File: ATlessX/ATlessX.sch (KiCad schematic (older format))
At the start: 13 parts, among them U1 74LS74, U2 74LS14

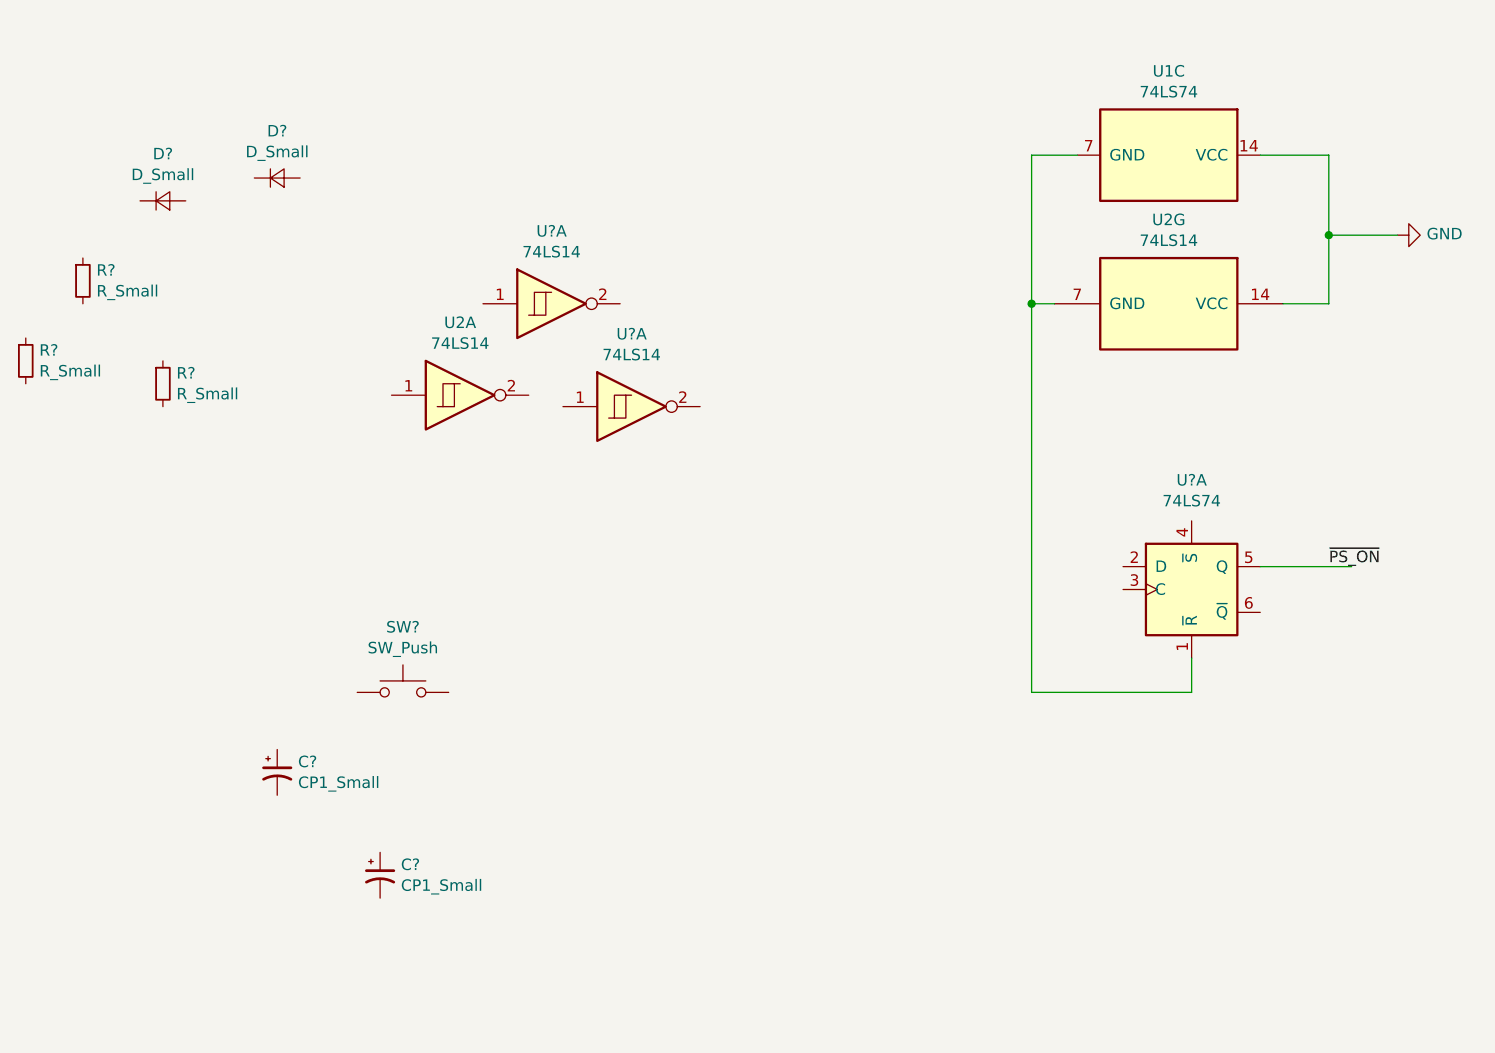
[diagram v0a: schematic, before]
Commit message: More of the circuit done
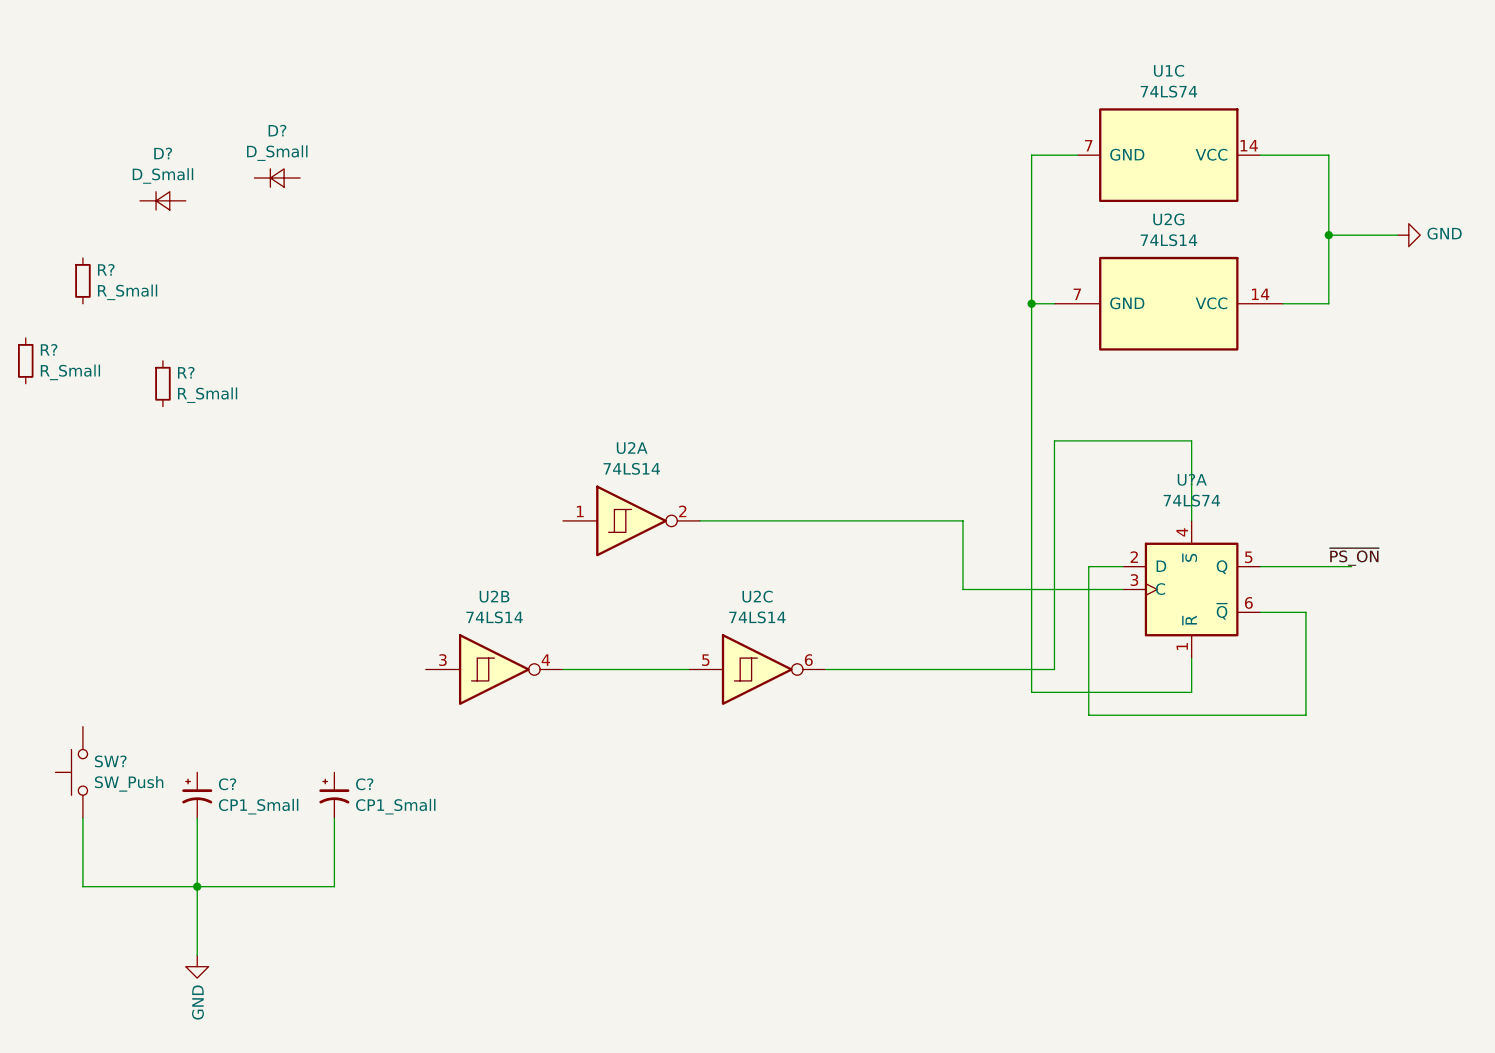
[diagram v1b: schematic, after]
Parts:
- gave numbers to parts that had none: 1
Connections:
- wire segments 12 -> 31
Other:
- moved on the sheet: C?, SW?, U2A
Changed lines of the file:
@@
 $Comp
 L 74xx:74LS14 U2
-U 1 1 5DD82518
-P 2500 2300
-F 0 "U2" H 2500 2617 50  0000 C CNN
-F 1 "74LS14" H 2500 2526 50  0000 C CNN
-F 2 "" H 2500 2300 50  0001 C CNN
-F 3 "http://www.ti.com/lit/gpn/sn74LS14" H 2500 2300 50  0001 C CNN
-	1    2500 2300
+U 2 1 5DD82518
+P 2650 3500
+F 0 "U2" H 2650 3817 50  0000 C CNN
+F 1 "74LS14" H 2650 3726 50  0000 C CNN
+F 2 "" H 2650 3500 50  0001 C CNN
+F 3 "http://www.ti.com/lit/gpn/sn74LS14" H 2650 3500 50  0001 C CNN
+	2    2650 3500
 	1    0    0    -1
 $EndComp
@@
 L Switch:SW_Push SW?
 U 1 1 5DD82728
-P 2250 3600
-F 0 "SW?" H 2250 3885 50  0000 C CNN
-F 1 "SW_Push" H 2250 3794 50  0000 C CNN
-F 2 "" H 2250 3800 50  0001 C CNN
-F 3 "~" H 2250 3800 50  0001 C CNN
-	1    2250 3600
-	1    0    0    -1
+P 850 3950
+F 0 "SW?" V 896 3902 50  0000 R CNN
+F 1 "SW_Push" V 805 3902 50  0000 R CNN
+F 2 "" H 850 4150 50  0001 C CNN
+F 3 "~" H 850 4150 50  0001 C CNN
+	1    850  3950
+	0    -1   -1   0
 $EndComp
 $Comp
 L Device:CP1_Small C?
 U 1 1 5DD82992
-P 2150 4400
-F 0 "C?" H 2241 4446 50  0000 L CNN
-F 1 "CP1_Small" H 2241 4355 50  0000 L CNN
-F 2 "" H 2150 4400 50  0001 C CNN
-F 3 "~" H 2150 4400 50  0001 C CNN
-	1    2150 4400
-	1    0    0    -1
-$EndComp
-$Comp
-L 74xx:74LS14 U?
+P 1950 4050
+F 0 "C?" H 2041 4096 50  0000 L CNN
+F 1 "CP1_Small" H 2041 4005 50  0000 L CNN
+F 2 "" H 1950 4050 50  0001 C CNN
+F 3 "~" H 1950 4050 50  0001 C CNN
+	1    1950 4050
+	1    0    0    -1
+$EndComp
+$Comp
+L 74xx:74LS14 U2
 U 1 1 5DD82CD4
-P 2900 1900
-F 0 "U?" H 2900 2217 50  0000 C CNN
-F 1 "74LS14" H 2900 2126 50  0000 C CNN
-F 2 "" H 2900 1900 50  0001 C CNN
-F 3 "http://www.ti.com/lit/gpn/sn74LS14" H 2900 1900 50  0001 C CNN
-	1    2900 1900
-	1    0    0    -1
-$EndComp
-$Comp
-L 74xx:74LS14 U?
-U 1 1 5DD82D12
-P 3250 2350
-F 0 "U?" H 3250 2667 50  0000 C CNN
-F 1 "74LS14" H 3250 2576 50  0000 C CNN
-F 2 "" H 3250 2350 50  0001 C CNN
-F 3 "http://www.ti.com/lit/gpn/sn74LS14" H 3250 2350 50  0001 C CNN
-	1    3250 2350
+P 3250 2850
+F 0 "U2" H 3250 3167 50  0000 C CNN
+F 1 "74LS14" H 3250 3076 50  0000 C CNN
+F 2 "" H 3250 2850 50  0001 C CNN
+F 3 "http://www.ti.com/lit/gpn/sn74LS14" H 3250 2850 50  0001 C CNN
+	1    3250 2850
+	1    0    0    -1
+$EndComp
+$Comp
+L 74xx:74LS14 U2
+U 3 1 5DD82D12
+P 3800 3500
+F 0 "U2" H 3800 3817 50  0000 C CNN
+F 1 "74LS14" H 3800 3726 50  0000 C CNN
+F 2 "" H 3800 3500 50  0001 C CNN
+F 3 "http://www.ti.com/lit/gpn/sn74LS14" H 3800 3500 50  0001 C CNN
+	3    3800 3500
 	1    0    0    -1
 $EndComp
@@
 L Device:CP1_Small C?
 U 1 1 5DD82E48
-P 1700 3950
-F 0 "C?" H 1791 3996 50  0000 L CNN
-F 1 "CP1_Small" H 1791 3905 50  0000 L CNN
-F 2 "" H 1700 3950 50  0001 C CNN
-F 3 "~" H 1700 3950 50  0001 C CNN
-	1    1700 3950
-	1    0    0    -1
-$EndComp
+P 1350 4050
+F 0 "C?" H 1441 4096 50  0000 L CNN
+F 1 "CP1_Small" H 1441 4005 50  0000 L CNN
+F 2 "" H 1350 4050 50  0001 C CNN
+F 3 "~" H 1350 4050 50  0001 C CNN
+	1    1350 4050
+	1    0    0    -1
+$EndComp
+Wire Wire Line
+	2950 3500 3500 3500
+Wire Wire Line
+	4100 3500 5100 3500
+Wire Wire Line
+	5100 3500 5100 2500
+Wire Wire Line
+	5100 2500 5700 2500
+Wire Wire Line
+	5700 2500 5700 2850
+Wire Wire Line
+	3550 2850 4700 2850
+Wire Wire Line
+	4700 2850 4700 3150
+Wire Wire Line
+	4700 3150 5400 3150
+Wire Wire Line
+	5400 3050 5250 3050
+Wire Wire Line
+	5250 3050 5250 3700
+Wire Wire Line
+	5250 3700 6200 3700
+Wire Wire Line
+	6200 3700 6200 3250
+Wire Wire Line
+	6200 3250 6000 3250
+Wire Wire Line
+	850  4150 850  4450
+Wire Wire Line
+	850  4450 1350 4450
+Wire Wire Line
+	1950 4450 1950 4150
+Wire Wire Line
+	1350 4150 1350 4450
+Connection ~ 1350 4450
+Wire Wire Line
+	1350 4450 1950 4450
+$Comp
+L power:GND #PWR?
+U 1 1 5DD84F2D
+P 1350 4750
+F 0 "#PWR?" H 1350 4500 50  0001 C CNN
+F 1 "GND" V 1355 4622 50  0000 R CNN
+F 2 "" H 1350 4750 50  0001 C CNN
+F 3 "" H 1350 4750 50  0001 C CNN
+	1    1350 4750
+	1    0    0    -1
+$EndComp
+Wire Wire Line
+	1350 4450 1350 4750
 $EndSCHEMATC

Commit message: Update schematic
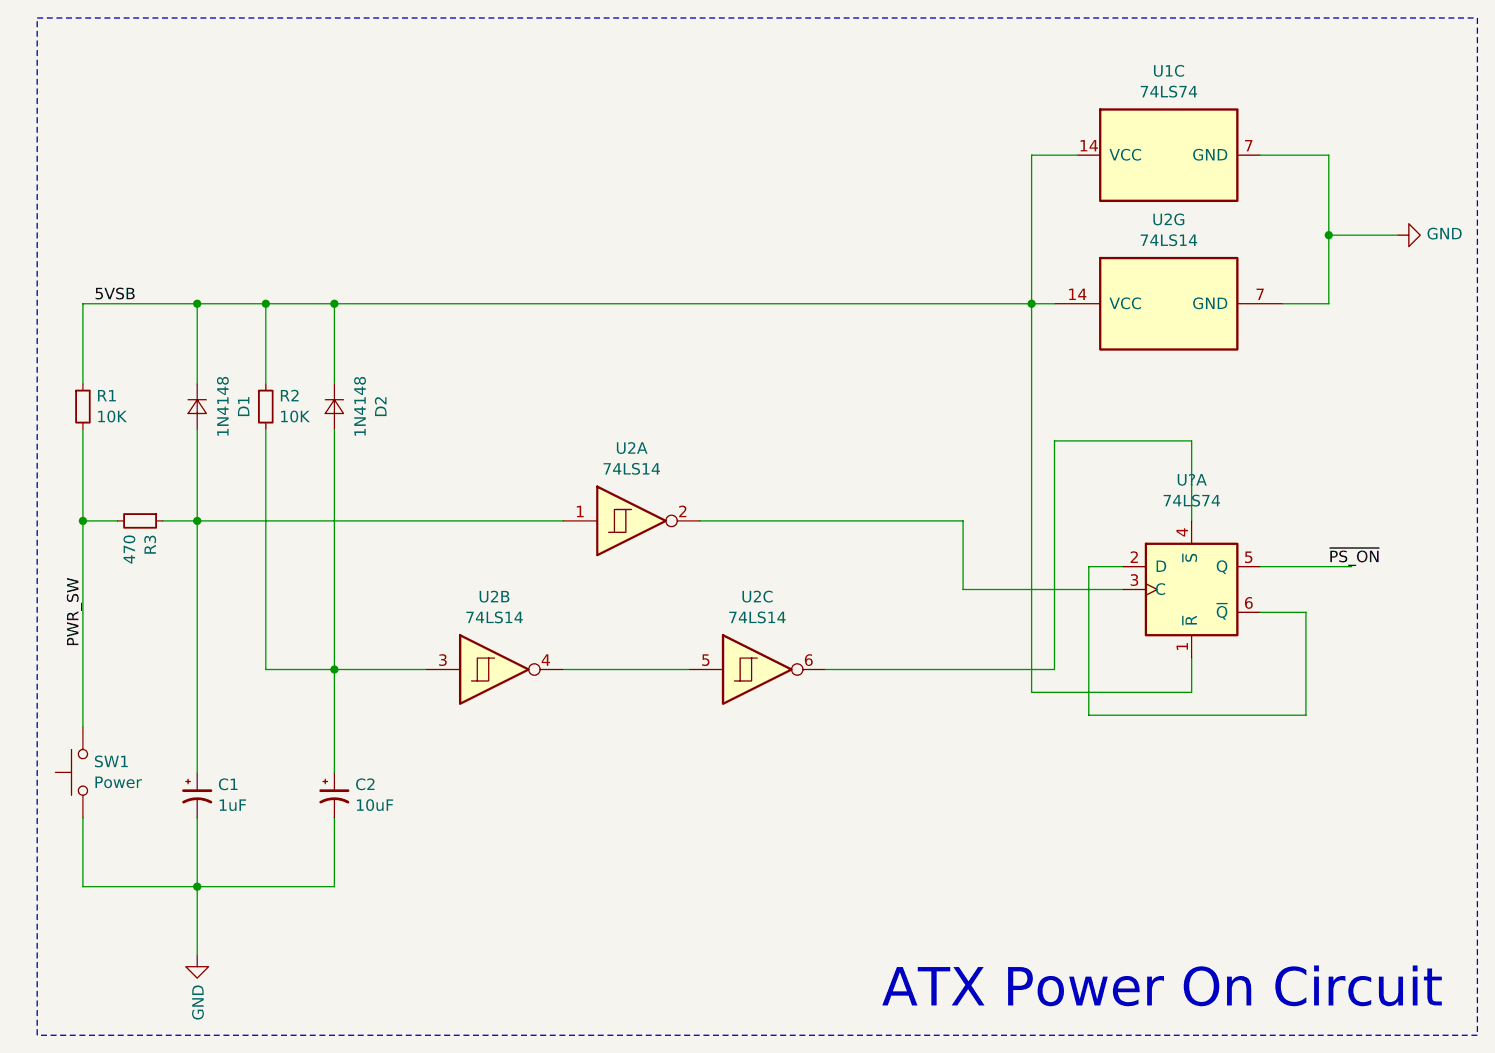
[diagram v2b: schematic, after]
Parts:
- C1: renamed from C?; value CP1_Small -> 1uF
- C2: renamed from C?; value CP1_Small -> 10uF
- D1, D2: renamed from D?; value D_Small -> 1N4148
- R1, R2: renamed from R?; value R_Small -> 10K
- R3: renamed from R?; value R_Small -> 470
- SW1: renamed from SW?; value SW_Push -> Power
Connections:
- net labels added: 5VSB, PWR_SW
- wire segments 31 -> 51
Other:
- note added: "ATX Power On Circuit"
- moved on the sheet: D1, D2, R1, R2, R3
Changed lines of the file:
@@
 F 3 "74xx/74hc_hct74.pdf" H 5600 1250 50  0001 C CNN
 	3    5600 1250
-	0    1    1    0
+	0    -1   1    0
 $EndComp
 $Comp
@@
 F 3 "http://www.ti.com/lit/gpn/sn74LS14" H 5600 1900 50  0001 C CNN
 	7    5600 1900
-	0    1    1    0
+	0    -1   1    0
 $EndComp
 Wire Wire Line
@@
 Connection ~ 5000 1900
 $Comp
-L Device:D_Small D?
+L Device:D_Small D1
 U 1 1 5DD82675
-P 1200 1450
-F 0 "D?" H 1200 1655 50  0000 C CNN
-F 1 "D_Small" H 1200 1564 50  0000 C CNN
-F 2 "" V 1200 1450 50  0001 C CNN
-F 3 "~" V 1200 1450 50  0001 C CNN
-	1    1200 1450
-	1    0    0    -1
-$EndComp
-$Comp
-L Device:R_Small R?
+P 1350 2350
+F 0 "D1" H 1350 2555 50  0000 C CNN
+F 1 "1N4148" H 1350 2464 50  0000 C CNN
+F 2 "" V 1350 2350 50  0001 C CNN
+F 3 "~" V 1350 2350 50  0001 C CNN
+	1    1350 2350
+	0    1    1    0
+$EndComp
+$Comp
+L Device:R_Small R3
 U 1 1 5DD827BB
-P 850 1800
-F 0 "R?" H 909 1846 50  0000 L CNN
-F 1 "R_Small" H 909 1755 50  0000 L CNN
-F 2 "" H 850 1800 50  0001 C CNN
-F 3 "~" H 850 1800 50  0001 C CNN
-	1    850  1800
-	1    0    0    -1
-$EndComp
-$Comp
-L Switch:SW_Push SW?
+P 1100 2850
+F 0 "R3" H 1159 2896 50  0000 L CNN
+F 1 "470" H 1159 2805 50  0000 L CNN
+F 2 "" H 1100 2850 50  0001 C CNN
+F 3 "~" H 1100 2850 50  0001 C CNN
+	1    1100 2850
+	0    1    1    0
+$EndComp
+$Comp
+L Switch:SW_Push SW1
 U 1 1 5DD82728
 P 850 3950
-F 0 "SW?" V 896 3902 50  0000 R CNN
-F 1 "SW_Push" V 805 3902 50  0000 R CNN
+F 0 "SW1" V 896 3902 50  0000 R CNN
+F 1 "Power" V 805 3902 50  0000 R CNN
 F 2 "" H 850 4150 50  0001 C CNN
 F 3 "~" H 850 4150 50  0001 C CNN
@@
 $EndComp
 $Comp
-L Device:CP1_Small C?
+L Device:CP1_Small C2
 U 1 1 5DD82992
 P 1950 4050
-F 0 "C?" H 2041 4096 50  0000 L CNN
-F 1 "CP1_Small" H 2041 4005 50  0000 L CNN
+F 0 "C2" H 2041 4096 50  0000 L CNN
+F 1 "10uF" H 2041 4005 50  0000 L CNN
 F 2 "" H 1950 4050 50  0001 C CNN
 F 3 "~" H 1950 4050 50  0001 C CNN
@@
 $EndComp
 $Comp
-L Device:R_Small R?
+L Device:R_Small R1
 U 1 1 5DD82D7E
-P 600 2150
-F 0 "R?" H 659 2196 50  0000 L CNN
-F 1 "R_Small" H 659 2105 50  0000 L CNN
-F 2 "" H 600 2150 50  0001 C CNN
-F 3 "~" H 600 2150 50  0001 C CNN
-	1    600  2150
-	1    0    0    -1
-$EndComp
-$Comp
-L Device:R_Small R?
+P 850 2350
+F 0 "R1" H 909 2396 50  0000 L CNN
+F 1 "10K" H 909 2305 50  0000 L CNN
+F 2 "" H 850 2350 50  0001 C CNN
+F 3 "~" H 850 2350 50  0001 C CNN
+	1    850  2350
+	1    0    0    -1
+$EndComp
+$Comp
+L Device:R_Small R2
 U 1 1 5DD82DBA
-P 1200 2250
-F 0 "R?" H 1259 2296 50  0000 L CNN
-F 1 "R_Small" H 1259 2205 50  0000 L CNN
-F 2 "" H 1200 2250 50  0001 C CNN
-F 3 "~" H 1200 2250 50  0001 C CNN
-	1    1200 2250
-	1    0    0    -1
-$EndComp
-$Comp
-L Device:D_Small D?
+P 1650 2350
+F 0 "R2" H 1709 2396 50  0000 L CNN
+F 1 "10K" H 1709 2305 50  0000 L CNN
+F 2 "" H 1650 2350 50  0001 C CNN
+F 3 "~" H 1650 2350 50  0001 C CNN
+	1    1650 2350
+	1    0    0    -1
+$EndComp
+$Comp
+L Device:D_Small D2
 U 1 1 5DD82DEF
-P 1700 1350
-F 0 "D?" H 1700 1555 50  0000 C CNN
-F 1 "D_Small" H 1700 1464 50  0000 C CNN
-F 2 "" V 1700 1350 50  0001 C CNN
-F 3 "~" V 1700 1350 50  0001 C CNN
-	1    1700 1350
-	1    0    0    -1
-$EndComp
-$Comp
-L Device:CP1_Small C?
+P 1950 2350
+F 0 "D2" H 1950 2555 50  0000 C CNN
+F 1 "1N4148" H 1950 2464 50  0000 C CNN
+F 2 "" V 1950 2350 50  0001 C CNN
+F 3 "~" V 1950 2350 50  0001 C CNN
+	1    1950 2350
+	0    1    1    0
+$EndComp
+$Comp
+L Device:CP1_Small C1
 U 1 1 5DD82E48
 P 1350 4050
-F 0 "C?" H 1441 4096 50  0000 L CNN
-F 1 "CP1_Small" H 1441 4005 50  0000 L CNN
+F 0 "C1" H 1441 4096 50  0000 L CNN
+F 1 "1uF" H 1441 4005 50  0000 L CNN
 F 2 "" H 1350 4050 50  0001 C CNN
 F 3 "~" H 1350 4050 50  0001 C CNN
@@
 Wire Wire Line
 	1350 4450 1350 4750
+Wire Wire Line
+	1650 2450 1650 3500
+Wire Wire Line
+	1650 3500 1950 3500
+Wire Wire Line
+	1950 3950 1950 3500
+Connection ~ 1950 3500
+Wire Wire Line
+	1950 3500 2350 3500
+Wire Wire Line
+	1950 3500 1950 2450
+Wire Wire Line
+	1350 2450 1350 2850
+Wire Wire Line
+	2950 2850 1350 2850
+Connection ~ 1350 2850
+Wire Wire Line
+	1350 2850 1350 3950
+Wire Wire Line
+	1200 2850 1350 2850
+Wire Wire Line
+	850  3750 850  2850
+Wire Wire Line
+	850  2850 1000 2850
+Wire Wire Line
+	850  2850 850  2450
+Connection ~ 850  2850
+Wire Wire Line
+	850  2250 850  1900
+Wire Wire Line
+	850  1900 1350 1900
+Wire Wire Line
+	1950 2250 1950 1900
+Connection ~ 1950 1900
+Wire Wire Line
+	1950 1900 5000 1900
+Wire Wire Line
+	1650 2250 1650 1900
+Connection ~ 1650 1900
+Wire Wire Line
+	1650 1900 1950 1900
+Wire Wire Line
+	1350 2250 1350 1900
+Connection ~ 1350 1900
+Wire Wire Line
+	1350 1900 1650 1900
+Text Label 900  1900 0    50   ~ 0
+5VSB
+Text Label 850  3400 1    50   ~ 0
+PWR_SW
+Wire Notes Line
+	650  650  6950 650
+Wire Notes Line
+	6950 650  6950 5100
+Wire Notes Line
+	6950 5100 650  5100
+Wire Notes Line
+	650  5100 650  650
+Text Notes 6800 5000 2    168  ~ 0
+ATX Power On Circuit
 $EndSCHEMATC
